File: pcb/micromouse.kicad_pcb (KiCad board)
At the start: 2 copper layers, 50 x 71 mm, 60 parts, among them J1 B2B-PH-K-S, J10 PINHD_1x4_Female, J12 PINHD_1x5_Female, J13 PINHD_1x5_Male, J14 PINHD_1x5_Male, J15 PINHD_1x2_Female, J16 PINHD_1x2_Male, J19 PINHD_1x4_Female, J2 B2B-PH-K-S, J3 B6B-ZR, J4 B6B-ZR, J5 PINHD_1x7_Female, J6 PINHD_1x7_Female, J7 PINHD_1x5_Female, J8 PINHD_1x7_Female, J9 PINHD_1x7_Female, M1 Left, M2 Right, M3 KDB0305HA3-00C1J, SW2 SW_DIP_x04, U1 AZ1117-3.3, U2 L293DD, U3 STM32F411RETx, U4 ICM-42688-P, Y1 25 MHz 10 pF, Y2 32.768 kHz 7 pF

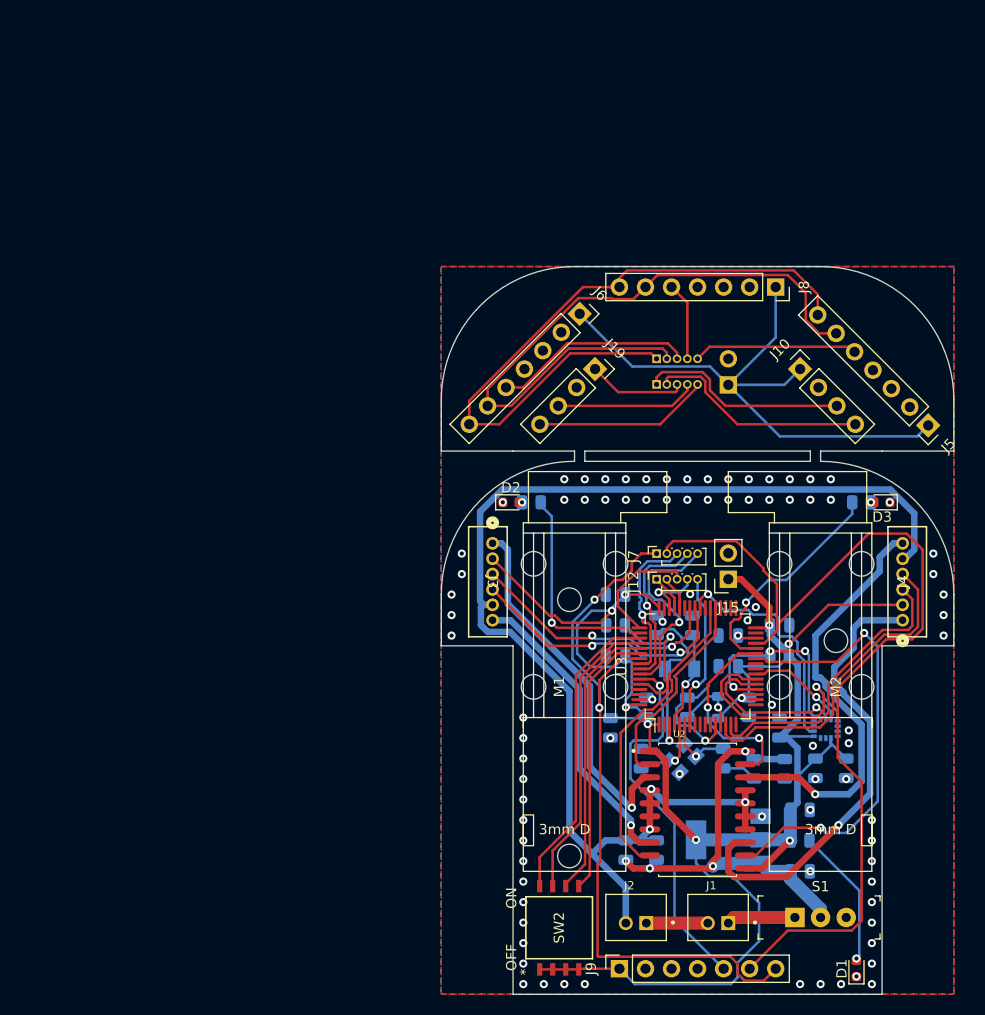
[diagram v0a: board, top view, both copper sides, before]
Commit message: Add files via upload
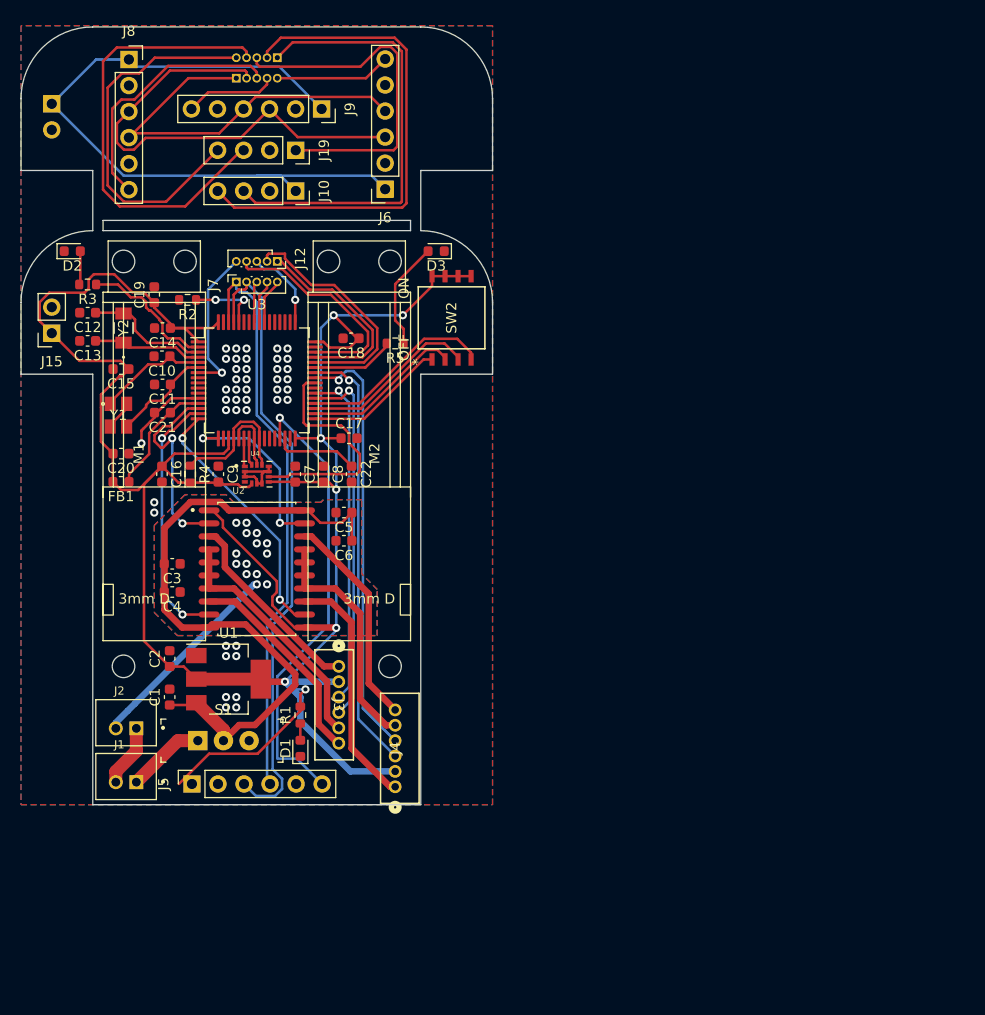
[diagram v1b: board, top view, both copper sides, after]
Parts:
- removed M3: KDB0305HA3-00C1J, custom:KDB0305HA3-00C1J
- C1, C10, C11, C12, C13, C14, C15, C16, C17, C18, C19, C2, C20, C21, C22, C3, C4, C5, C6, C7, C8, C9: footprint Capacitor_SMD:C_0805_2012Metric -> Capacitor_SMD:C_0603_1608Metric; moved to F.Cu
- FB1: footprint Inductor_SMD:L_0805_2012Metric -> Inductor_SMD:L_0603_1608Metric; moved to F.Cu
- J5, J6, J8, J9: value PINHD_1x7_Female -> PINHD_1x6_Female; footprint Connector_PinSocket_2.54mm:PinSocket_1x07_P2.54mm_Vertical -> Connector_PinSocket_2.54mm:PinSocket_1x06_P2.54mm_Vertical
- NT2, U1, U4, Y1, Y2: moved to F.Cu
- R1, R2, R3, R4, R5: footprint Resistor_SMD:R_0805_2012Metric -> Resistor_SMD:R_0603_1608Metric; moved to F.Cu
- moved J9 88.8 mm to (153.3, 73.6), turned to -90 degrees
- moved J5 79.9 mm to (140.7, 139.5), turned to 90 degrees
- moved J16 71.5 mm to (127.0, 73.1), turned to 180 degrees
- moved J15 70.2 mm to (127.0, 95.5)
- moved C9 67.6 mm to (143.2, 109.2)
- moved J8 66.9 mm to (134.5, 68.8), turned to 0 degrees
- moved C20 66.1 mm to (133.8, 107.2), turned to 180 degrees
- moved C11 65.8 mm to (137.8, 100.5), turned to 180 degrees
- moved C13 65.2 mm to (130.5, 96.2), turned to 180 degrees
- moved Y1 64.4 mm to (133.5, 103.5), turned to 0 degrees
- moved C1 63.8 mm to (138.5, 131.0), turned to 90 degrees
- moved Y2 63.6 mm to (134.0, 95.0), turned to 90 degrees
- moved C12 63.3 mm to (130.5, 93.5), turned to 180 degrees
- moved C2 63.2 mm to (138.5, 127.2), turned to 90 degrees
- moved FB1 62.3 mm to (133.8, 110.0), turned to 180 degrees
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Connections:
- C10 pad 1: GND -> OSC_IN
- C10 pad 2: OSC_IN -> GND
- C20 pad 1: +3.3V -> GND
- C20 pad 2: GND -> +3.3V
- C5 pad 2: GND -> GND1
- C6 pad 2: GND -> GND1
- C7 pad 1: +3.3V -> GND
- C7 pad 2: GND -> +3.3V
- C8 pad 1: +3.3V -> GND
- C8 pad 2: GND -> +3.3V
- C9 pad 1: +3.3V -> GND
- C9 pad 2: GND -> +3.3V
- FB1 pad 1: +3.3V -> +3.3VA
- FB1 pad 2: +3.3VA -> +3.3V
- J5 pad 1: /Breakout Board/+3.3V -> +3.3V
- J5 pad 2: unconnected-(J5-Pad2) -> GND
- J5 pad 3: GND -> /SCL
- J5 pad 4: unconnected-(J5-Pad4) -> /SDA
- J5 pad 5: /Breakout Board/SHDN3 -> unconnected-(J5-Pad5)
- J5 pad 6: /Breakout Board/SCL -> /SHDN4
- J6 pad 2: unconnected-(J6-Pad2) -> GND
- J6 pad 3: GND -> /Breakout Board/SCL
- J6 pad 4: unconnected-(J6-Pad4) -> /Breakout Board/SDA
- J6 pad 5: /Breakout Board/SHDN1 -> unconnected-(J6-Pad5)
- J6 pad 6: /Breakout Board/SCL -> /Breakout Board/SHDN3
- J7 pad 1: I2C2_SDA -> /SDA
- J7 pad 2: I2C2_SCL -> /SCL
- J8 pad 2: unconnected-(J8-Pad2) -> GND
- J8 pad 3: GND -> /Breakout Board/SCL
- J8 pad 4: unconnected-(J8-Pad4) -> /Breakout Board/SDA
- J8 pad 5: /Breakout Board/SHDN2 -> unconnected-(J8-Pad5)
- J8 pad 6: /Breakout Board/SCL -> /Breakout Board/SHDN1
- J9 pad 1: +3.3V -> /Breakout Board/+3.3V
- J9 pad 2: unconnected-(J9-Pad2) -> GND
- J9 pad 3: GND -> /Breakout Board/SCL
- J9 pad 4: unconnected-(J9-Pad4) -> /Breakout Board/SDA
- J9 pad 5: /SHDN4 -> unconnected-(J9-Pad5)
- J9 pad 6: I2C2_SCL -> /Breakout Board/SHDN2
- R1 pad 1: +3.3V -> Net-(D1-A)
- R1 pad 2: Net-(D1-A) -> +3.3V
- R3 pad 1: /LED1 -> Net-(D2-A)
- R3 pad 2: Net-(D2-A) -> /LED1
- R4 pad 1: /IMU/SPI_CS -> SPI_CS_BYPASS
- R5 pad 1: /LED2 -> Net-(D3-A)
- R5 pad 2: Net-(D3-A) -> /LED2
- SW2 pad 1: +3.3V -> DEBUG1
- SW2 pad 2: +3.3V -> DEBUG2
- SW2 pad 3: +3.3V -> DEBUG3
- SW2 pad 4: +3.3V -> DEBUG4
- SW2 pad 5: DEBUG4 -> +3.3V
- SW2 pad 6: DEBUG3 -> +3.3V
- SW2 pad 7: DEBUG2 -> +3.3V
- SW2 pad 8: DEBUG1 -> +3.3V
- U3 pad 14: ER1 -> HL1
- U3 pad 15: ER2 -> HL2
- U3 pad 16: FAN_PWM -> HR1
- U3 pad 17: FAN_TACH -> HR2
- U3 pad 2: unconnected-(U3-PC13-Pad2) -> /LED1
- U3 pad 20: /IMU/SPI_CS -> SPI_CS_BYPASS
- U3 pad 21: /IMU/SPI_SCLK -> SPI_SCLK_BYPASS
- U3 pad 24: unconnected-(U3-PC4-Pad24) -> SPI_SCLK_BYPASS
- U3 pad 25: unconnected-(U3-PC5-Pad25) -> SPI_CS_BYPASS
- U3 pad 26: HR1 -> unconnected-(U3-PB0-Pad26)
- U3 pad 27: HR2 -> unconnected-(U3-PB1-Pad27)
- U3 pad 28: /LED2 -> unconnected-(U3-PB2-Pad28)
- U3 pad 29: I2C2_SCL -> /SHDN4
- U3 pad 33: SPI2_NSS -> DEBUG1
- U3 pad 34: SPI2_SCK -> DEBUG2
- U3 pad 35: SPI2_MISO -> DEBUG3
- U3 pad 36: SPI2_MOSI -> DEBUG4
- U3 pad 37: HL1 -> EL1
- U3 pad 38: HL2 -> EL2
- U3 pad 41: EL1 -> ER1
- U3 pad 42: EL2 -> ER2
- U3 pad 43: unconnected-(U3-PA10-Pad43) -> /LED2
- U3 pad 50: /LED1 -> unconnected-(U3-PA15-Pad50)
- U3 pad 51: DEBUG1 -> unconnected-(U3-PC10-Pad51)
- U3 pad 52: DEBUG2 -> unconnected-(U3-PC11-Pad52)
- U3 pad 53: DEBUG3 -> unconnected-(U3-PC12-Pad53)
- U3 pad 54: DEBUG4 -> unconnected-(U3-PD2-Pad54)
- U3 pad 55: I2C2_SDA -> /SHDN3
- U3 pad 56: /SHDN1 -> /SHDN2
- U3 pad 57: /SHDN2 -> /SHDN1
- U3 pad 58: /SHDN3 -> unconnected-(U3-PB6-Pad58)
- U3 pad 59: /SHDN4 -> unconnected-(U3-PB7-Pad59)
- U3 pad 61: I2C1_SCL -> /SCL
- U3 pad 62: I2C1_SDA -> /SDA
- U4 pad 12: /IMU/SPI_CS -> SPI_CS_BYPASS
- U4 pad 13: /IMU/SPI_SCLK -> SPI_SCLK_BYPASS
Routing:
- net I2C2_SCL: track 94.6 -> 0.00 mm
- net I2C2_SDA: track 72.1 -> 0.00 mm, vias 2 -> 0
- net /SCL: track 0.00 -> 61.7 mm
- net GND1: track 124.2 -> 64.0 mm, vias 3 -> 14
- net /SDA: track 0.00 -> 56.6 mm
- net +3.3V: track 189.2 -> 242.0 mm, vias 9 -> 7
- net /Breakout Board/SWDIO: track 13.8 -> 44.5 mm
- net /Breakout Board/USART_TX: track 21.6 -> 49.5 mm
- net /Breakout Board/SDA: track 66.8 -> 40.1 mm
- net /Breakout Board/SWCLK: track 9.59 -> 34.6 mm
- net +BATT: track 41.0 -> 64.7 mm, vias 4 -> 0
- net /Breakout Board/USART_RX: track 20.5 -> 43.8 mm
- net MR2: track 45.0 -> 23.5 mm, vias 1 -> 0
- net MR1: track 41.9 -> 21.0 mm, vias 1 -> 0
- net /IMU/SPI_SD0: track 23.1 -> 2.76 mm, vias 1 -> 0
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- added copper zone on B.Cu, net GND1
- added copper zone on F.Cu, net GND1
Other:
- board size 50 x 71 mm -> 46 x 75.9 mm
- board text removed: "<- HAT Connector"
